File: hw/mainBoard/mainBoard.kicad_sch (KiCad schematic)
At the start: 0 parts

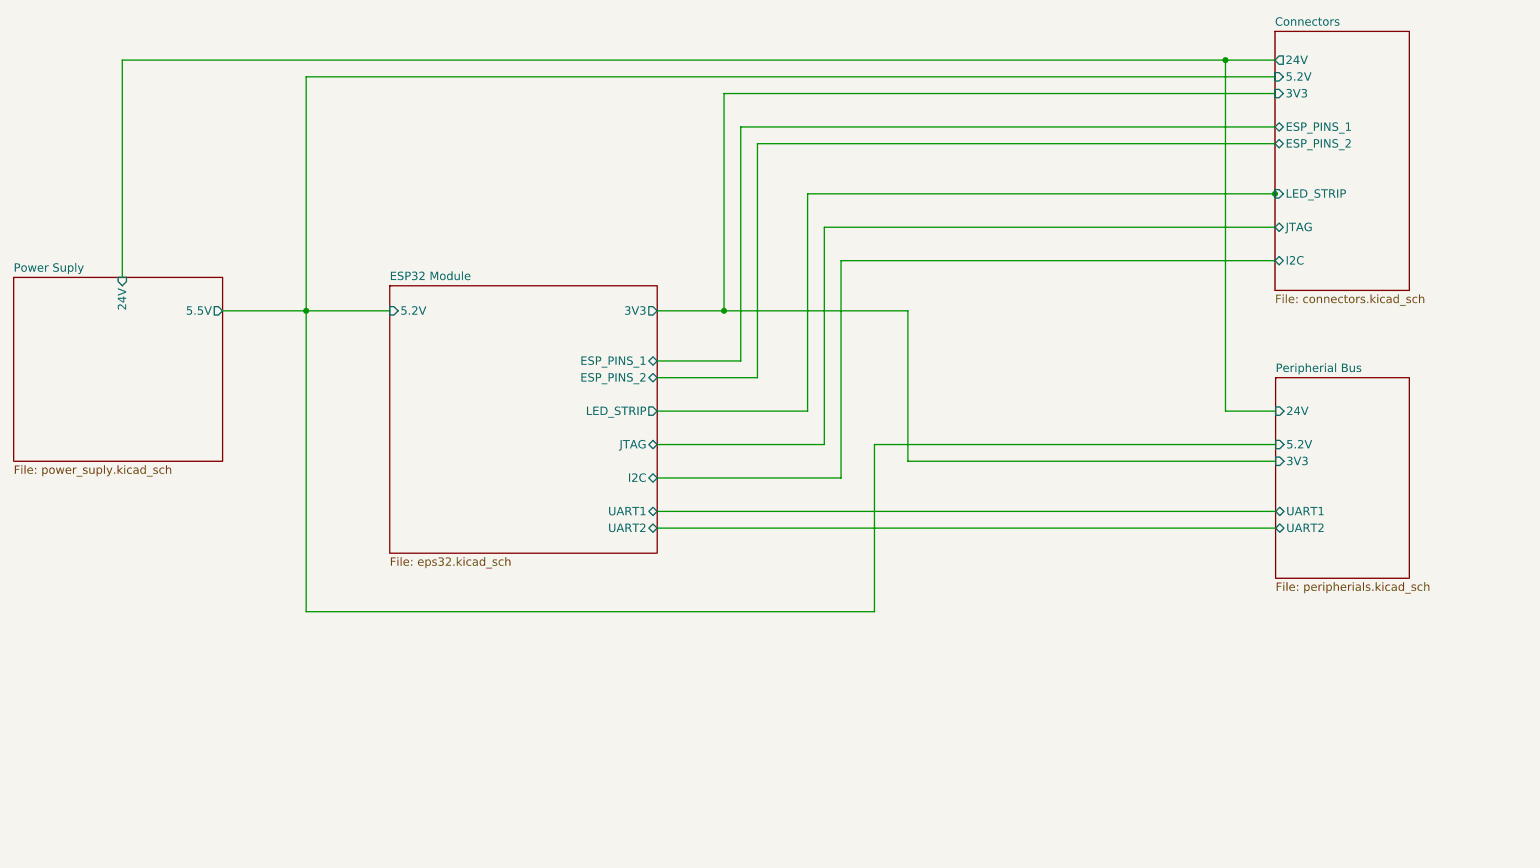
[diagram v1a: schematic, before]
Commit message: nejaky hw + teorie + desky
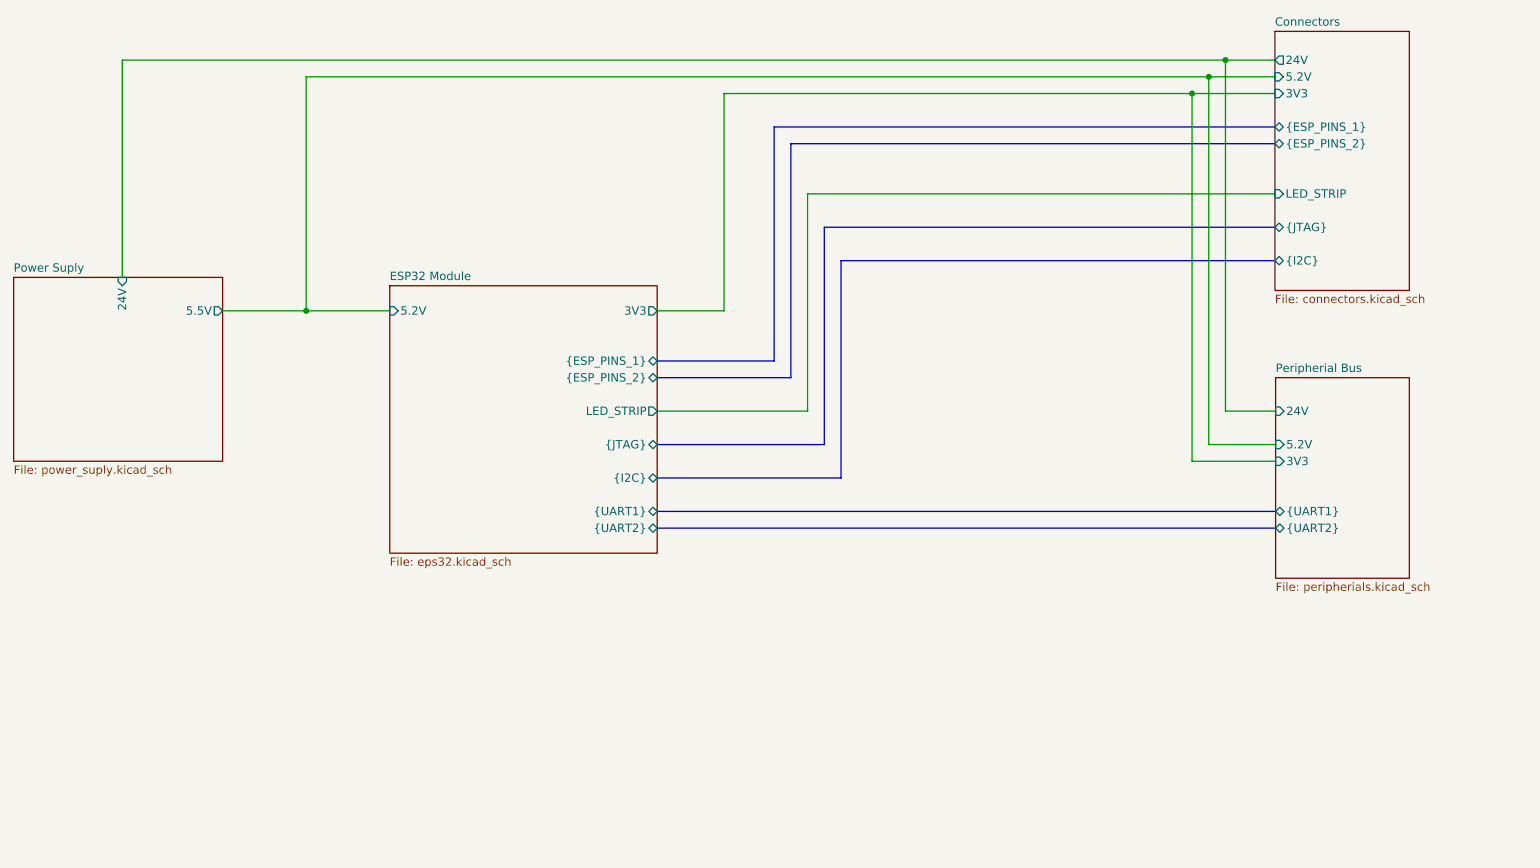
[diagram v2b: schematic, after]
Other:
- sheet Connectors ports: added {ESP_PINS_1}, {ESP_PINS_2}, {I2C}, {JTAG}; removed ESP_PINS_1, ESP_PINS_2, I2C, JTAG
- sheet ESP32 Module ports: added {ESP_PINS_1}, {ESP_PINS_2}, {I2C}, {JTAG}, {UART1}, {UART2}; removed ESP_PINS_1, ESP_PINS_2, I2C, JTAG, UART1, UART2
- sheet Peripherial Bus ports: added {UART1}, {UART2}; removed UART1, UART2
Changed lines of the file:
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@@
   (junction (at 215.9 35.56) (diameter 0) (color 0 0 0 0)
   )
-  (junction (at 139.7 73.66) (diameter 0) (color 0 0 0 0)
-  )
-  (junction (at 223.4202 55.88) (diameter 0) (color 0 0 0 0)
+  (junction (at 210.82 40.64) (diameter 0) (color 0 0 0 0)
   )
   (junction (at 76.2 73.66) (diameter 0) (color 0 0 0 0)
   )
-  (wire (pts (xy 76.2 119.38) (xy 162.56 119.38))
-    (stroke (width 0) (type default))
+  (junction (at 213.36 38.1) (diameter 0) (color 0 0 0 0)
   )
   (wire (pts (xy 76.2 73.66) (xy 76.2 38.1))
@@
     (stroke (width 0) (type default))
   )
-  (wire (pts (xy 129.54 81.28) (xy 142.24 81.28))
-    (stroke (width 0) (type default))
-  )
-  (wire (pts (xy 162.56 93.98) (xy 223.52 93.98))
+  (bus (pts (xy 154.94 60.96) (xy 223.4202 60.96))
+    (stroke (width 0) (type default))
+  )
+  (bus (pts (xy 149.86 83.82) (xy 149.86 48.26))
+    (stroke (width 0) (type default))
+  )
+  (bus (pts (xy 147.32 81.28) (xy 147.32 45.72))
     (stroke (width 0) (type default))
   )
@@
     (stroke (width 0) (type default))
   )
-  (wire (pts (xy 139.7 40.64) (xy 223.4202 40.64))
-    (stroke (width 0) (type default))
-  )
-  (wire (pts (xy 76.2 38.1) (xy 223.4202 38.1))
+  (wire (pts (xy 139.7 40.64) (xy 210.82 40.64))
+    (stroke (width 0) (type default))
+  )
+  (wire (pts (xy 76.2 38.1) (xy 213.36 38.1))
     (stroke (width 0) (type default))
   )
@@
     (stroke (width 0) (type default))
   )
-  (wire (pts (xy 129.54 104.14) (xy 223.52 104.14))
-    (stroke (width 0) (type default))
-  )
-  (wire (pts (xy 167.64 96.52) (xy 223.52 96.52))
-    (stroke (width 0) (type default))
-  )
-  (wire (pts (xy 142.24 45.72) (xy 223.4202 45.72))
+  (bus (pts (xy 157.48 66.04) (xy 223.4202 66.04))
+    (stroke (width 0) (type default))
+  )
+  (bus (pts (xy 129.54 106.68) (xy 223.52 106.68))
+    (stroke (width 0) (type default))
+  )
+  (bus (pts (xy 147.32 45.72) (xy 223.4202 45.72))
+    (stroke (width 0) (type default))
+  )
+  (bus (pts (xy 149.86 48.26) (xy 223.4202 48.26))
     (stroke (width 0) (type default))
   )
@@
     (stroke (width 0) (type default))
   )
-  (wire (pts (xy 129.54 83.82) (xy 144.78 83.82))
-    (stroke (width 0) (type default))
-  )
-  (wire (pts (xy 162.56 119.38) (xy 162.56 93.98))
+  (bus (pts (xy 129.54 99.06) (xy 157.48 99.06))
     (stroke (width 0) (type default))
   )
@@
     (stroke (width 0) (type default))
   )
-  (wire (pts (xy 76.2 73.66) (xy 76.2 119.38))
-    (stroke (width 0) (type default))
-  )
-  (wire (pts (xy 157.48 99.06) (xy 157.48 66.04))
-    (stroke (width 0) (type default))
-  )
-  (wire (pts (xy 223.4202 55.88) (xy 223.52 55.88))
-    (stroke (width 0) (type default))
-  )
-  (wire (pts (xy 129.54 99.06) (xy 157.48 99.06))
-    (stroke (width 0) (type default))
-  )
-  (wire (pts (xy 129.54 93.98) (xy 154.94 93.98))
-    (stroke (width 0) (type default))
-  )
-  (wire (pts (xy 142.24 81.28) (xy 142.24 45.72))
+  (bus (pts (xy 129.54 104.14) (xy 223.52 104.14))
+    (stroke (width 0) (type default))
+  )
+  (wire (pts (xy 210.82 96.52) (xy 210.82 40.64))
+    (stroke (width 0) (type default))
+  )
+  (bus (pts (xy 129.54 83.82) (xy 149.86 83.82))
+    (stroke (width 0) (type default))
+  )
+  (bus (pts (xy 129.54 81.28) (xy 147.32 81.28))
     (stroke (width 0) (type default))
   )
@@
     (stroke (width 0) (type default))
   )
-  (wire (pts (xy 157.48 66.04) (xy 223.4202 66.04))
-    (stroke (width 0) (type default))
-  )
-  (wire (pts (xy 144.78 48.26) (xy 223.4202 48.26))
+  (wire (pts (xy 213.36 38.1) (xy 223.4202 38.1))
     (stroke (width 0) (type default))
   )
@@
     (stroke (width 0) (type default))
   )
-  (wire (pts (xy 167.64 73.66) (xy 167.64 96.52))
-    (stroke (width 0) (type default))
-  )
-  (wire (pts (xy 139.7 73.66) (xy 167.64 73.66))
+  (wire (pts (xy 223.52 96.52) (xy 210.82 96.52))
     (stroke (width 0) (type default))
   )
@@
     (stroke (width 0) (type default))
   )
-  (wire (pts (xy 144.78 83.82) (xy 144.78 48.26))
-    (stroke (width 0) (type default))
-  )
   (wire (pts (xy 215.9 35.56) (xy 215.9 88.9))
     (stroke (width 0) (type default))
   )
-  (wire (pts (xy 154.94 60.96) (xy 223.4202 60.96))
-    (stroke (width 0) (type default))
-  )
-  (wire (pts (xy 129.54 106.68) (xy 223.52 106.68))
+  (bus (pts (xy 129.54 93.98) (xy 154.94 93.98))
+    (stroke (width 0) (type default))
+  )
+  (bus (pts (xy 157.48 99.06) (xy 157.48 66.04))
+    (stroke (width 0) (type default))
+  )
+  (wire (pts (xy 213.36 93.98) (xy 213.36 38.1))
     (stroke (width 0) (type default))
   )
@@
     (stroke (width 0) (type default))
   )
-  (wire (pts (xy 154.94 93.98) (xy 154.94 60.96))
+  (wire (pts (xy 223.52 93.98) (xy 213.36 93.98))
+    (stroke (width 0) (type default))
+  )
+  (wire (pts (xy 210.82 40.64) (xy 223.4202 40.64))
+    (stroke (width 0) (type default))
+  )
+  (bus (pts (xy 154.94 93.98) (xy 154.94 60.96))
     (stroke (width 0) (type default))
   )
@@
       (effects (font (size 1.27 1.27)) (justify left top))
     )
-    (pin "UART2" bidirectional (at 223.52 106.68 180)
-      (effects (font (size 1.27 1.27)) (justify left))
-    )
-    (pin "UART1" bidirectional (at 223.52 104.14 180)
-      (effects (font (size 1.27 1.27)) (justify left))
-    )
     (pin "3V3" input (at 223.52 96.52 180)
       (effects (font (size 1.27 1.27)) (justify left))
@@
     )
     (pin "24V" input (at 223.52 88.9 180)
+      (effects (font (size 1.27 1.27)) (justify left))
+    )
+    (pin "{UART1}" bidirectional (at 223.52 104.14 180)
+      (effects (font (size 1.27 1.27)) (justify left))
+    )
+    (pin "{UART2}" bidirectional (at 223.52 106.68 180)
       (effects (font (size 1.27 1.27)) (justify left))
     )
@@
       (effects (font (size 1.27 1.27)) (justify left top))
     )
-    (pin "ESP_PINS_2" bidirectional (at 129.54 83.82 0)
-      (effects (font (size 1.27 1.27)) (justify right))
-    )
-    (pin "ESP_PINS_1" bidirectional (at 129.54 81.28 0)
-      (effects (font (size 1.27 1.27)) (justify right))
-    )
-    (pin "UART1" bidirectional (at 129.54 104.14 0)
-      (effects (font (size 1.27 1.27)) (justify right))
-    )
-    (pin "UART2" bidirectional (at 129.54 106.68 0)
-      (effects (font (size 1.27 1.27)) (justify right))
-    )
-    (pin "JTAG" bidirectional (at 129.54 93.98 0)
-      (effects (font (size 1.27 1.27)) (justify right))
-    )
-    (pin "I2C" bidirectional (at 129.54 99.06 0)
-      (effects (font (size 1.27 1.27)) (justify right))
-    )
     (pin "3V3" output (at 129.54 73.66 0)
       (effects (font (size 1.27 1.27)) (justify right))
@@
     )
     (pin "LED_STRIP" output (at 129.54 88.9 0)
+      (effects (font (size 1.27 1.27)) (justify right))
+    )
+    (pin "{I2C}" bidirectional (at 129.54 99.06 0)
+      (effects (font (size 1.27 1.27)) (justify right))
+    )
+    (pin "{ESP_PINS_2}" bidirectional (at 129.54 83.82 0)
+      (effects (font (size 1.27 1.27)) (justify right))
+    )
+    (pin "{ESP_PINS_1}" bidirectional (at 129.54 81.28 0)
+      (effects (font (size 1.27 1.27)) (justify right))
+    )
+    (pin "{JTAG}" bidirectional (at 129.54 93.98 0)
+      (effects (font (size 1.27 1.27)) (justify right))
+    )
+    (pin "{UART2}" bidirectional (at 129.54 106.68 0)
+      (effects (font (size 1.27 1.27)) (justify right))
+    )
+    (pin "{UART1}" bidirectional (at 129.54 104.14 0)
       (effects (font (size 1.27 1.27)) (justify right))
     )
@@
       (effects (font (size 1.27 1.27)) (justify left top))
     )
-    (pin "JTAG" bidirectional (at 223.4202 60.96 180)
-      (effects (font (size 1.27 1.27)) (justify left))
-    )
-    (pin "ESP_PINS_2" bidirectional (at 223.4202 48.26 180)
-      (effects (font (size 1.27 1.27)) (justify left))
-    )
-    (pin "ESP_PINS_1" bidirectional (at 223.4202 45.72 180)
-      (effects (font (size 1.27 1.27)) (justify left))
-    )
-    (pin "I2C" bidirectional (at 223.4202 66.04 180)
-      (effects (font (size 1.27 1.27)) (justify left))
-    )
     (pin "3V3" input (at 223.4202 40.64 180)
       (effects (font (size 1.27 1.27)) (justify left))
@@
       (effects (font (size 1.27 1.27)) (justify left))
     )
+    (pin "{I2C}" bidirectional (at 223.4202 66.04 180)
+      (effects (font (size 1.27 1.27)) (justify left))
+    )
+    (pin "{ESP_PINS_2}" bidirectional (at 223.4202 48.26 180)
+      (effects (font (size 1.27 1.27)) (justify left))
+    )
+    (pin "{ESP_PINS_1}" bidirectional (at 223.4202 45.72 180)
+      (effects (font (size 1.27 1.27)) (justify left))
+    )
+    (pin "{JTAG}" bidirectional (at 223.4202 60.96 180)
+      (effects (font (size 1.27 1.27)) (justify left))
+    )
